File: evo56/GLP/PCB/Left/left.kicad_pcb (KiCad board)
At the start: 2 copper layers, 139.9 x 114.8 mm, 82 parts

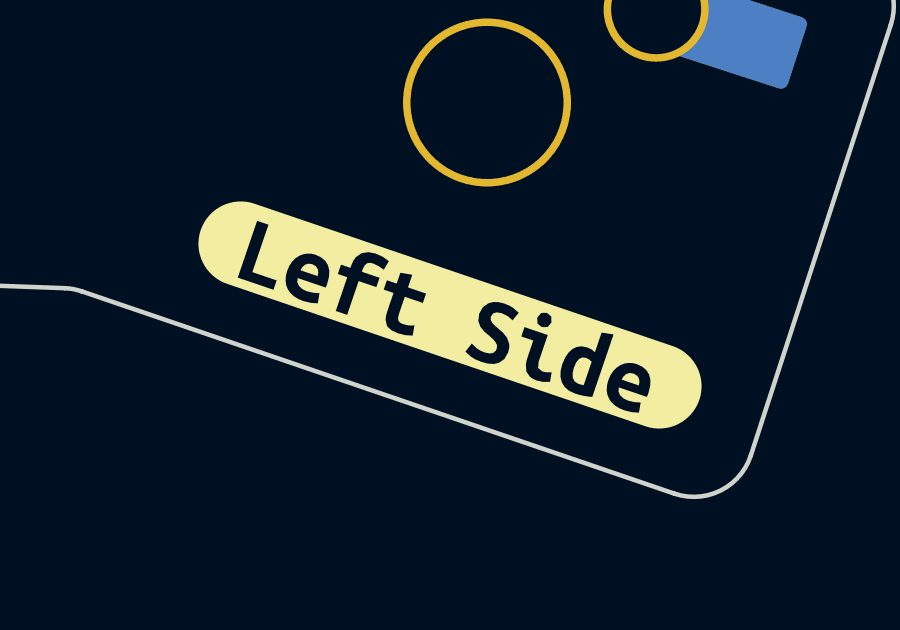
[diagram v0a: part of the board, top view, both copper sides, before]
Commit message: yep
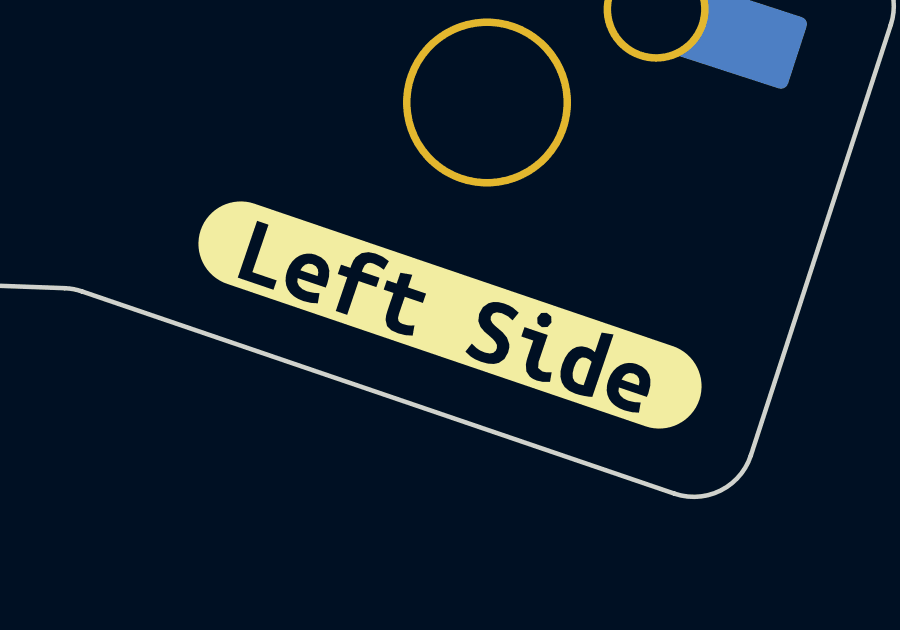
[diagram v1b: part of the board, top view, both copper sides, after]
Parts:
- removed kibuzzard-67FD52C7: G***, kibuzzard-67FD52C7
- added kibuzzard-67FD9A83: G***, kibuzzard-67FD9A83, F.Cu at (164.6, 163.2)
